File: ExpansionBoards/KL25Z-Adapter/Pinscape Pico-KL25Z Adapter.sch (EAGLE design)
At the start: 17 parts, among them IC1 PCA9555APW,118, IC2 PCA9555APW,118, IC3 LIS3DHTR, IC30 ADS1115IDGSR, SW1 TS-1187A-B-A-B

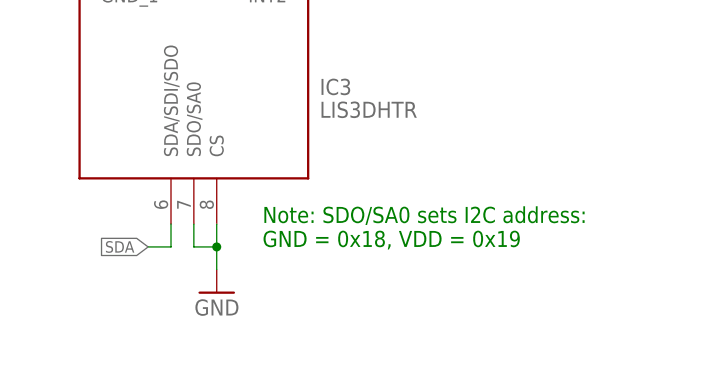
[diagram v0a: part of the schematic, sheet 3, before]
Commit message: bug fixes
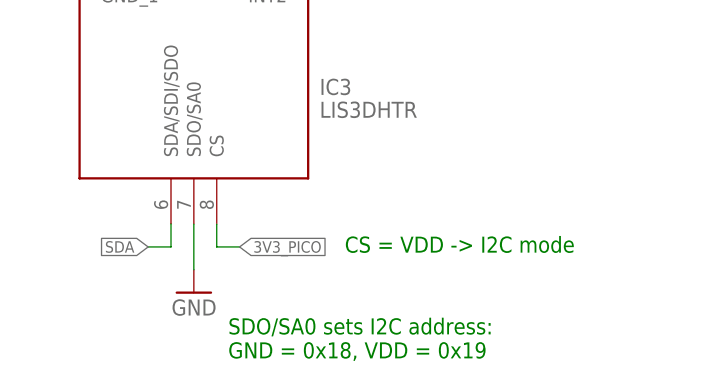
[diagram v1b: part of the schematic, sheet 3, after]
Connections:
- net 3V3_PICO: now also IC3.CS
- net GND: no longer IC3.CS
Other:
- note added: "CS = VDD -> I2C mode"
- note added: "SDO/SA0 sets I2C address: GND = 0x18, VDD = 0x19"
- note removed: "Note: SDO/SA0 sets I2C address: GND = 0x18, VDD = 0x19"
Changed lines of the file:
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@@
 <text x="7.62" y="73.66" size="2.54" layer="91">Accelerometer
 I2C address 0x18</text>
-<text x="71.12" y="12.7" size="1.778" layer="91">Note: SDO/SA0 sets I2C address:
+<text x="67.31" y="2.54" size="1.778" layer="91" align="center-left">SDO/SA0 sets I2C address:
 GND = 0x18, VDD = 0x19</text>
+<text x="80.264" y="12.954" size="1.778" layer="91" align="center-left">CS = VDD -&gt; I2C mode</text>
 </plain>
 <instances>
@@
 <attribute name="VALUE" x="77.47" y="27.94" size="1.778" layer="96" align="center-left"/>
 </instance>
-<instance part="GND42" gate="1" x="66.04" y="7.62" rot="MR0"/>
+<instance part="GND42" gate="1" x="63.5" y="7.62" rot="MR0"/>
 <instance part="GND51" gate="1" x="40.64" y="40.64" rot="MR90"/>
 <instance part="GND52" gate="1" x="86.36" y="43.18" rot="MR270"/>
@@
 <net name="GND" class="0">
 <segment>
-<pinref part="IC3" gate="G$1" pin="CS"/>
 <pinref part="GND42" gate="1" pin="GND"/>
-<wire x1="66.04" y1="15.24" x2="66.04" y2="12.7" width="0.1524" layer="91"/>
 <pinref part="IC3" gate="G$1" pin="SDO/SA0"/>
-<wire x1="66.04" y1="12.7" x2="66.04" y2="10.16" width="0.1524" layer="91"/>
-<wire x1="63.5" y1="15.24" x2="63.5" y2="12.7" width="0.1524" layer="91"/>
-<wire x1="63.5" y1="12.7" x2="66.04" y2="12.7" width="0.1524" layer="91"/>
-<junction x="66.04" y="12.7"/>
+<wire x1="63.5" y1="15.24" x2="63.5" y2="10.16" width="0.1524" layer="91"/>
 </segment>
 <segment>
@@
 <junction x="22.86" y="50.8"/>
 </segment>
+<segment>
+<pinref part="IC3" gate="G$1" pin="CS"/>
+<wire x1="66.04" y1="15.24" x2="66.04" y2="12.7" width="0.1524" layer="91"/>
+<wire x1="66.04" y1="12.7" x2="68.58" y2="12.7" width="0.1524" layer="91"/>
+<label x="68.58" y="12.7" size="1.27" layer="95" xref="yes"/>
+</segment>
 </net>
